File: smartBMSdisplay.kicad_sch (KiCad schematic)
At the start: 7 parts, among them J1 Conn_01x04_Male, J2 Conn_01x05_Male, Q1 BC547

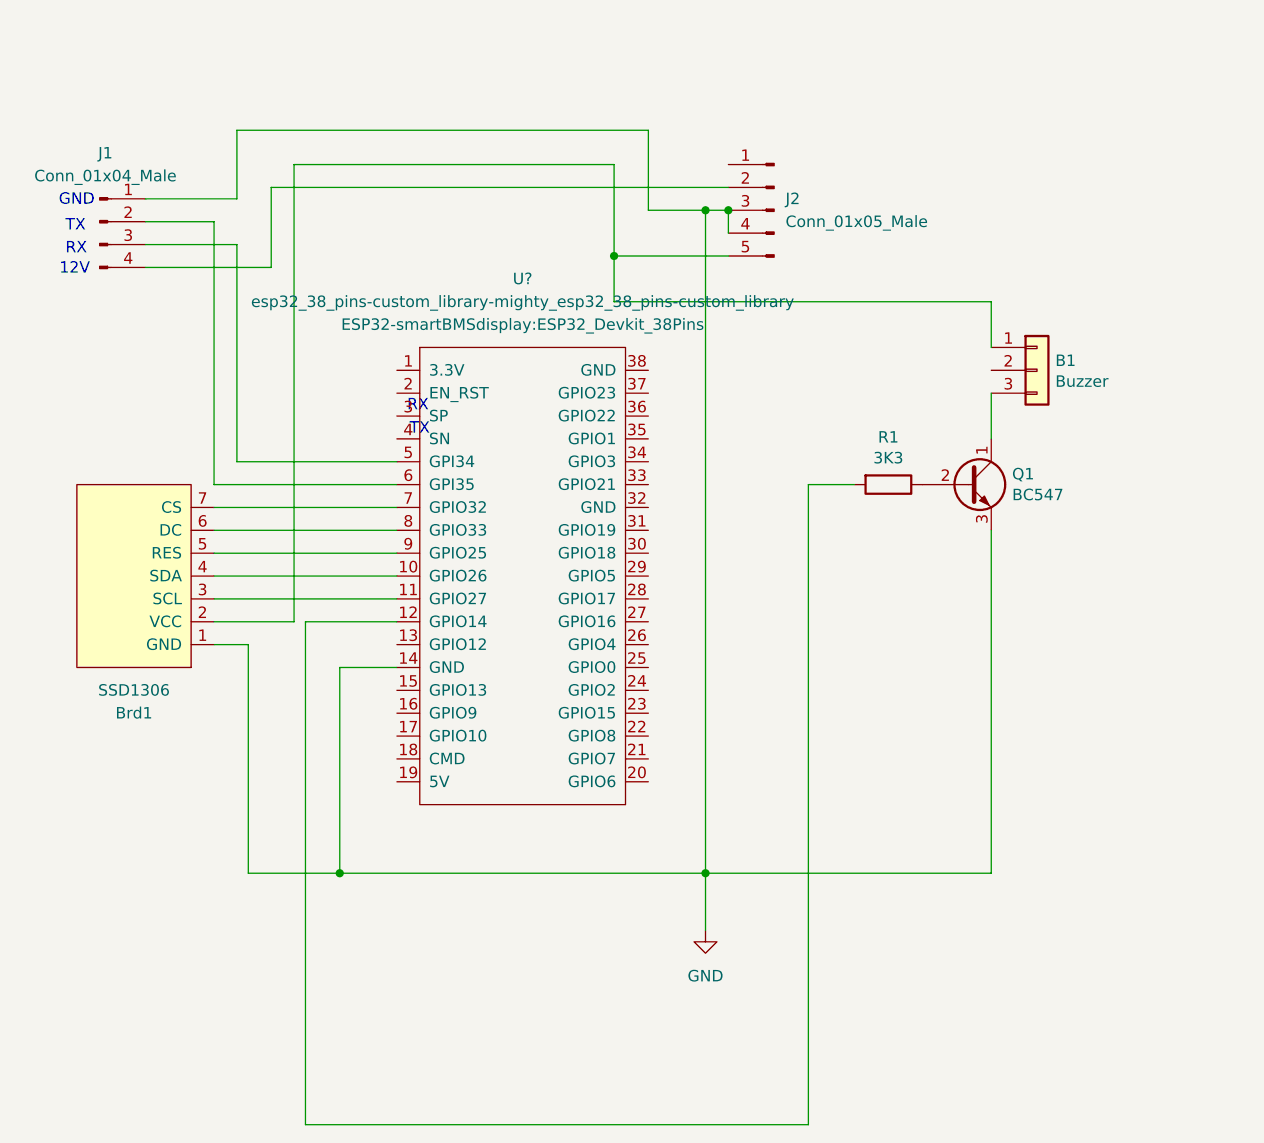
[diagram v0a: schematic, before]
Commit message: First working bluetooth version
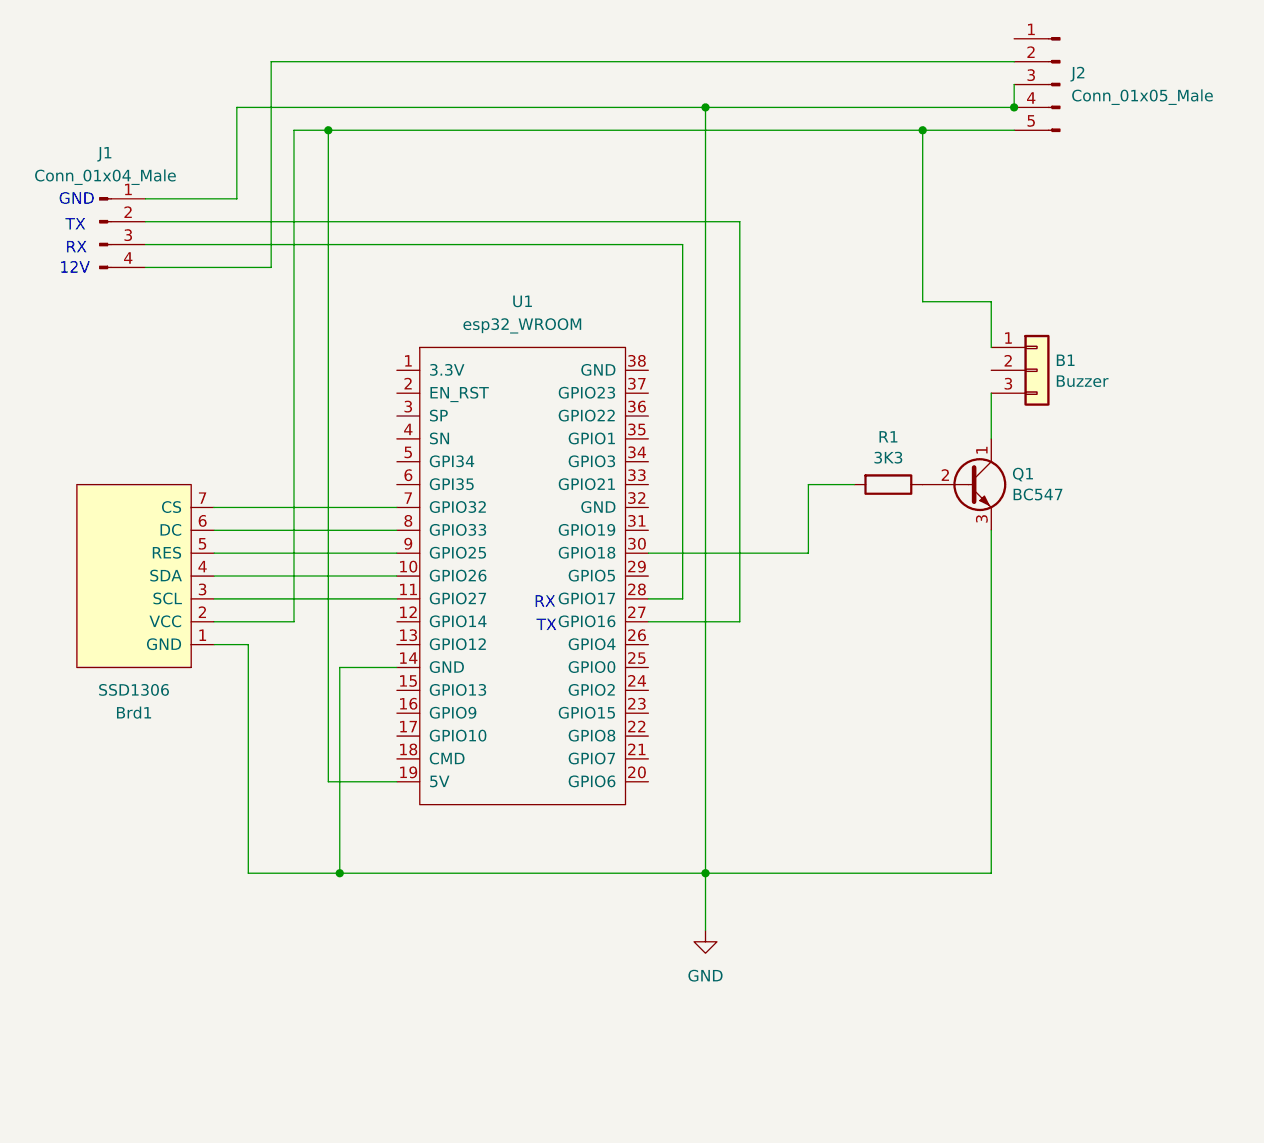
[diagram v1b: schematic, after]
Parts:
- U1: renamed from U?; value esp32_38_pins-custom_library-mighty_esp32_38_pins-custom_library -> esp32_WROOM
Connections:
- net at B1.1 (Pin_1), Brd1.2 (VCC), J2.5 (Pin_5): now also U1.19 (5V)
- net at R1.2: now also U1.30 (GPIO18); no longer U1.12 (GPIO14)
- net at J1.2 (Pin_2): now also U1.27 (GPIO16); no longer U1.6 (GPI35)
- net at J1.3 (Pin_3): now also U1.28 (GPIO17); no longer U1.5 (GPI34)
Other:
- moved on the sheet: J2
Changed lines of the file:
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@@
 (kicad_sch (version 20211123) (generator eeschema)
   (paper "A4")
+  (junction (at 179.07 58.42) (diameter 0) (color 0 0 0 0)
+  )
   (junction (at 104.14 143.51) (diameter 0) (color 0 0 0 0)
   )
-  (junction (at 144.78 69.85) (diameter 0) (color 0 0 0 0)
-  )
-  (junction (at 147.32 69.85) (diameter 0) (color 0 0 0 0)
+  (junction (at 144.78 58.42) (diameter 0) (color 0 0 0 0)
   )
   (junction (at 144.78 143.51) (diameter 0) (color 0 0 0 0)
   )
-  (junction (at 134.62 74.93) (diameter 0) (color 0 0 0 0)
+  (junction (at 102.87 60.96) (diameter 0) (color 0 0 0 0)
+  )
+  (junction (at 168.91 60.96) (diameter 0) (color 0 0 0 0)
   )
   (wire (pts (xy 176.53 143.51) (xy 144.78 143.51))
@@
     (stroke (width 0) (type default) (color 0 0 0 0))
   )
-  (wire (pts (xy 144.78 69.85) (xy 144.78 143.51))
-    (stroke (width 0) (type default) (color 0 0 0 0))
-  )
-  (wire (pts (xy 156.21 100.33) (xy 156.21 171.45))
-    (stroke (width 0) (type default) (color 0 0 0 0))
-  )
-  (wire (pts (xy 176.53 80.01) (xy 134.62 80.01))
+  (wire (pts (xy 144.78 58.42) (xy 144.78 143.51))
     (stroke (width 0) (type default) (color 0 0 0 0))
   )
@@
     (stroke (width 0) (type default) (color 0 0 0 0))
   )
-  (wire (pts (xy 138.43 69.85) (xy 144.78 69.85))
+  (wire (pts (xy 82.55 73.66) (xy 142.24 73.66))
     (stroke (width 0) (type default) (color 0 0 0 0))
   )
@@
     (stroke (width 0) (type default) (color 0 0 0 0))
   )
-  (wire (pts (xy 92.71 73.66) (xy 82.55 73.66))
-    (stroke (width 0) (type default) (color 0 0 0 0))
-  )
-  (wire (pts (xy 96.52 67.31) (xy 96.52 76.2))
-    (stroke (width 0) (type default) (color 0 0 0 0))
-  )
   (wire (pts (xy 90.17 107.95) (xy 110.49 107.95))
     (stroke (width 0) (type default) (color 0 0 0 0))
   )
+  (wire (pts (xy 102.87 60.96) (xy 168.91 60.96))
+    (stroke (width 0) (type default) (color 0 0 0 0))
+  )
+  (wire (pts (xy 168.91 60.96) (xy 168.91 80.01))
+    (stroke (width 0) (type default) (color 0 0 0 0))
+  )
   (wire (pts (xy 93.98 118.11) (xy 93.98 143.51))
     (stroke (width 0) (type default) (color 0 0 0 0))
   )
+  (wire (pts (xy 102.87 133.35) (xy 102.87 60.96))
+    (stroke (width 0) (type default) (color 0 0 0 0))
+  )
   (wire (pts (xy 90.17 110.49) (xy 110.49 110.49))
     (stroke (width 0) (type default) (color 0 0 0 0))
@@
     (stroke (width 0) (type default) (color 0 0 0 0))
   )
+  (wire (pts (xy 144.78 58.42) (xy 179.07 58.42))
+    (stroke (width 0) (type default) (color 0 0 0 0))
+  )
   (wire (pts (xy 82.55 68.58) (xy 92.71 68.58))
     (stroke (width 0) (type default) (color 0 0 0 0))
   )
-  (wire (pts (xy 90.17 100.33) (xy 110.49 100.33))
+  (wire (pts (xy 179.07 55.88) (xy 179.07 58.42))
     (stroke (width 0) (type default) (color 0 0 0 0))
   )
@@
     (stroke (width 0) (type default) (color 0 0 0 0))
   )
-  (wire (pts (xy 90.17 71.12) (xy 82.55 71.12))
-    (stroke (width 0) (type default) (color 0 0 0 0))
-  )
-  (wire (pts (xy 92.71 97.79) (xy 110.49 97.79))
-    (stroke (width 0) (type default) (color 0 0 0 0))
-  )
-  (wire (pts (xy 156.21 171.45) (xy 100.33 171.45))
-    (stroke (width 0) (type default) (color 0 0 0 0))
-  )
-  (wire (pts (xy 99.06 64.77) (xy 134.62 64.77))
-    (stroke (width 0) (type default) (color 0 0 0 0))
-  )
-  (wire (pts (xy 134.62 74.93) (xy 134.62 80.01))
-    (stroke (width 0) (type default) (color 0 0 0 0))
-  )
-  (wire (pts (xy 134.62 74.93) (xy 147.32 74.93))
-    (stroke (width 0) (type default) (color 0 0 0 0))
-  )
-  (wire (pts (xy 100.33 115.57) (xy 110.49 115.57))
+  (wire (pts (xy 82.55 71.12) (xy 148.59 71.12))
+    (stroke (width 0) (type default) (color 0 0 0 0))
+  )
+  (wire (pts (xy 179.07 53.34) (xy 96.52 53.34))
+    (stroke (width 0) (type default) (color 0 0 0 0))
+  )
+  (wire (pts (xy 156.21 100.33) (xy 156.21 107.95))
     (stroke (width 0) (type default) (color 0 0 0 0))
   )
@@
     (stroke (width 0) (type default) (color 0 0 0 0))
   )
-  (wire (pts (xy 100.33 171.45) (xy 100.33 115.57))
-    (stroke (width 0) (type default) (color 0 0 0 0))
-  )
   (wire (pts (xy 161.29 100.33) (xy 156.21 100.33))
     (stroke (width 0) (type default) (color 0 0 0 0))
   )
-  (wire (pts (xy 138.43 60.96) (xy 138.43 69.85))
-    (stroke (width 0) (type default) (color 0 0 0 0))
-  )
   (wire (pts (xy 90.17 115.57) (xy 99.06 115.57))
     (stroke (width 0) (type default) (color 0 0 0 0))
   )
-  (wire (pts (xy 92.71 73.66) (xy 92.71 97.79))
-    (stroke (width 0) (type default) (color 0 0 0 0))
-  )
-  (wire (pts (xy 134.62 64.77) (xy 134.62 74.93))
+  (wire (pts (xy 148.59 71.12) (xy 148.59 115.57))
+    (stroke (width 0) (type default) (color 0 0 0 0))
+  )
+  (wire (pts (xy 96.52 53.34) (xy 96.52 76.2))
+    (stroke (width 0) (type default) (color 0 0 0 0))
+  )
+  (wire (pts (xy 99.06 60.96) (xy 102.87 60.96))
+    (stroke (width 0) (type default) (color 0 0 0 0))
+  )
+  (wire (pts (xy 142.24 113.03) (xy 138.43 113.03))
+    (stroke (width 0) (type default) (color 0 0 0 0))
+  )
+  (wire (pts (xy 142.24 73.66) (xy 142.24 113.03))
     (stroke (width 0) (type default) (color 0 0 0 0))
   )
@@
     (stroke (width 0) (type default) (color 0 0 0 0))
   )
-  (wire (pts (xy 92.71 60.96) (xy 138.43 60.96))
-    (stroke (width 0) (type default) (color 0 0 0 0))
-  )
-  (wire (pts (xy 92.71 68.58) (xy 92.71 60.96))
-    (stroke (width 0) (type default) (color 0 0 0 0))
-  )
-  (wire (pts (xy 147.32 69.85) (xy 147.32 72.39))
-    (stroke (width 0) (type default) (color 0 0 0 0))
-  )
-  (wire (pts (xy 96.52 67.31) (xy 147.32 67.31))
+  (wire (pts (xy 168.91 60.96) (xy 179.07 60.96))
+    (stroke (width 0) (type default) (color 0 0 0 0))
+  )
+  (wire (pts (xy 92.71 58.42) (xy 144.78 58.42))
+    (stroke (width 0) (type default) (color 0 0 0 0))
+  )
+  (wire (pts (xy 92.71 68.58) (xy 92.71 58.42))
+    (stroke (width 0) (type default) (color 0 0 0 0))
+  )
+  (wire (pts (xy 156.21 107.95) (xy 138.43 107.95))
     (stroke (width 0) (type default) (color 0 0 0 0))
   )
@@
     (stroke (width 0) (type default) (color 0 0 0 0))
   )
-  (wire (pts (xy 99.06 115.57) (xy 99.06 64.77))
-    (stroke (width 0) (type default) (color 0 0 0 0))
-  )
-  (wire (pts (xy 144.78 69.85) (xy 147.32 69.85))
+  (wire (pts (xy 148.59 115.57) (xy 138.43 115.57))
+    (stroke (width 0) (type default) (color 0 0 0 0))
+  )
+  (wire (pts (xy 99.06 115.57) (xy 99.06 60.96))
     (stroke (width 0) (type default) (color 0 0 0 0))
   )
@@
     (stroke (width 0) (type default) (color 0 0 0 0))
   )
-  (wire (pts (xy 90.17 71.12) (xy 90.17 100.33))
-    (stroke (width 0) (type default) (color 0 0 0 0))
-  )
-  (text "RX" (at 111.6229 92.3683 0)
+  (wire (pts (xy 110.49 133.35) (xy 102.87 133.35))
+    (stroke (width 0) (type default) (color 0 0 0 0))
+  )
+  (wire (pts (xy 176.53 80.01) (xy 168.91 80.01))
+    (stroke (width 0) (type default) (color 0 0 0 0))
+  )
+  (text "RX" (at 125.73 114.3 0)
     (effects (font (size 1.27 1.27)) (justify left bottom))
   )
@@
     (effects (font (size 1.27 1.27)) (justify left bottom))
   )
-  (text "TX" (at 111.8964 94.967 0)
+  (text "TX" (at 126.0035 116.8987 0)
     (effects (font (size 1.27 1.27)) (justify left bottom))
   )
@@
     (effects (font (size 1.27 1.27)) (justify left bottom))
   )
-  (symbol (lib_id "Connector:Conn_01x05_Male") (at 152.4 69.85 0) (mirror y) (unit 1)
+  (symbol (lib_id "Connector:Conn_01x05_Male") (at 184.15 55.88 0) (mirror y) (unit 1)
     (in_bom yes) (on_board yes) (fields_autoplaced)
-    (property "Reference" "J2" (id 0) (at 153.67 68.5799 0)
+    (property "Reference" "J2" (id 0) (at 185.42 54.6099 0)
       (effects (font (size 1.27 1.27)) (justify right))
     )
-    (property "Value" "Conn_01x05_Male" (id 1) (at 153.67 71.1199 0)
+    (property "Value" "Conn_01x05_Male" (id 1) (at 185.42 57.1499 0)
       (effects (font (size 1.27 1.27)) (justify right))
     )
-    (property "Footprint" "Connector_PinHeader_2.54mm:PinHeader_1x05_P2.54mm_Vertical" (id 2) (at 152.4 69.85 0)
-      (effects (font (size 1.27 1.27)) hide)
-    )
-    (property "Datasheet" "~" (id 3) (at 152.4 69.85 0)
+    (property "Footprint" "Connector_PinHeader_2.54mm:PinHeader_1x05_P2.54mm_Vertical" (id 2) (at 184.15 55.88 0)
+      (effects (font (size 1.27 1.27)) hide)
+    )
+    (property "Datasheet" "~" (id 3) (at 184.15 55.88 0)
       (effects (font (size 1.27 1.27)) hide)
     )
@@
   (symbol (lib_id "esp32_38_pins-custom_library-mighty_esp32_38_pins-custom_library:esp32_38_pins-custom_library-mighty_esp32_38_pins-custom_library") (at 115.57 92.71 0) (unit 1)
     (in_bom yes) (on_board yes) (fields_autoplaced)
-    (property "Reference" "U?" (id 0) (at 124.46 77.47 0))
-    (property "Value" "esp32_38_pins-custom_library-mighty_esp32_38_pins-custom_library" (id 1) (at 124.46 80.01 0))
-    (property "Footprint" "ESP32-smartBMSdisplay:ESP32_Devkit_38Pins" (id 2) (at 124.46 82.55 0))
+    (property "Reference" "U1" (id 0) (at 124.46 80.01 0))
+    (property "Value" "esp32_WROOM" (id 1) (at 124.46 82.55 0))
+    (property "Footprint" "ESP32-smartBMSdisplay:ESP32_Devkit_38Pins" (id 2) (at 124.46 82.55 0)
+      (effects (font (size 1.27 1.27)) hide)
+    )
     (property "Datasheet" "" (id 3) (at 115.57 92.71 0))
     (pin "1")
@@
     )
     (path "/fa7cc373-1e9b-4a68-961b-8c9f216ebb9e"
-      (reference "U?") (unit 1) (value "esp32_38_pins-custom_library-mighty_esp32_38_pins-custom_library") (footprint "ESP32-smartBMSdisplay:ESP32_Devkit_38Pins")
-    )
-  )
+      (reference "U1") (unit 1) (value "esp32_WROOM") (footprint "ESP32-smartBMSdisplay:ESP32_Devkit_38Pins")
+    )
+  )
